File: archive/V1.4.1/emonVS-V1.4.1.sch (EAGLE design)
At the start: 47 parts, among them J7 RJ45 Jack, J8 TERMINAL_BLOCK_2P, J9 TERMINAL_BLOCK_5P, M1 275VAC, M2 275VAC, M3 275VAC, T1 ZMPT101B, T2 ZMPT101B, T3 ZMPT101B

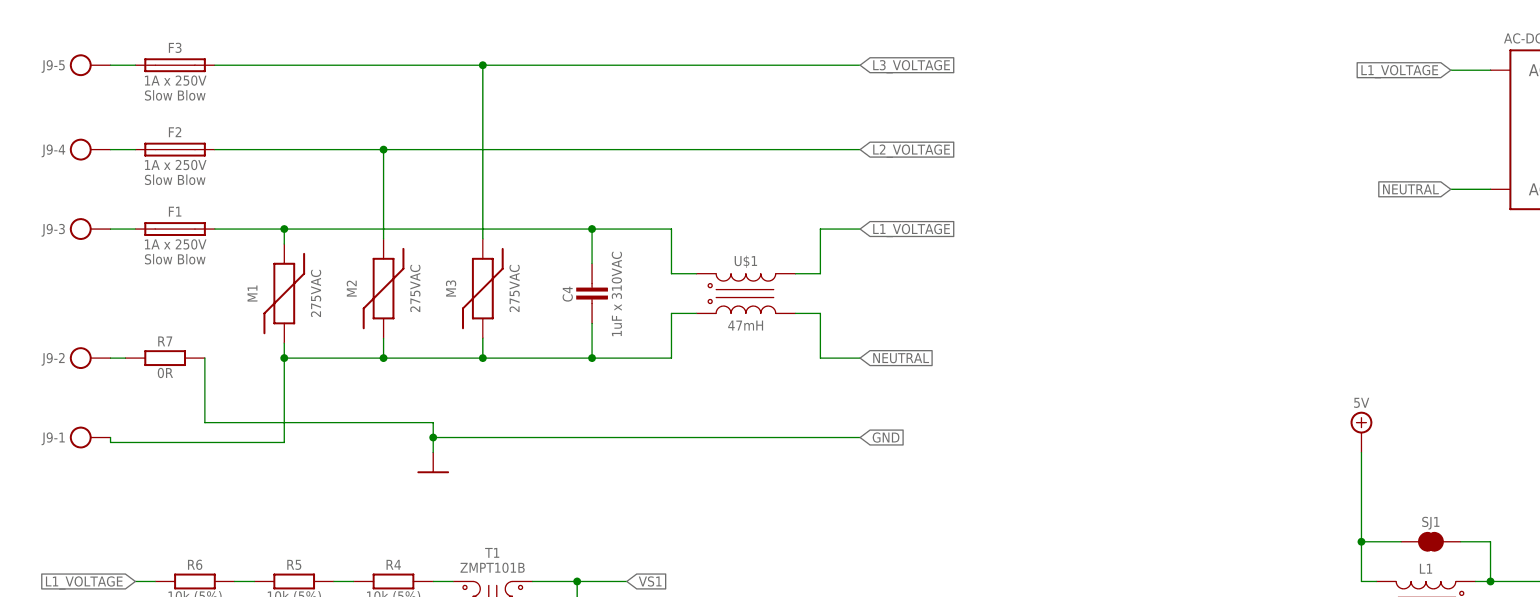
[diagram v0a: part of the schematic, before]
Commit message: 1.4.2
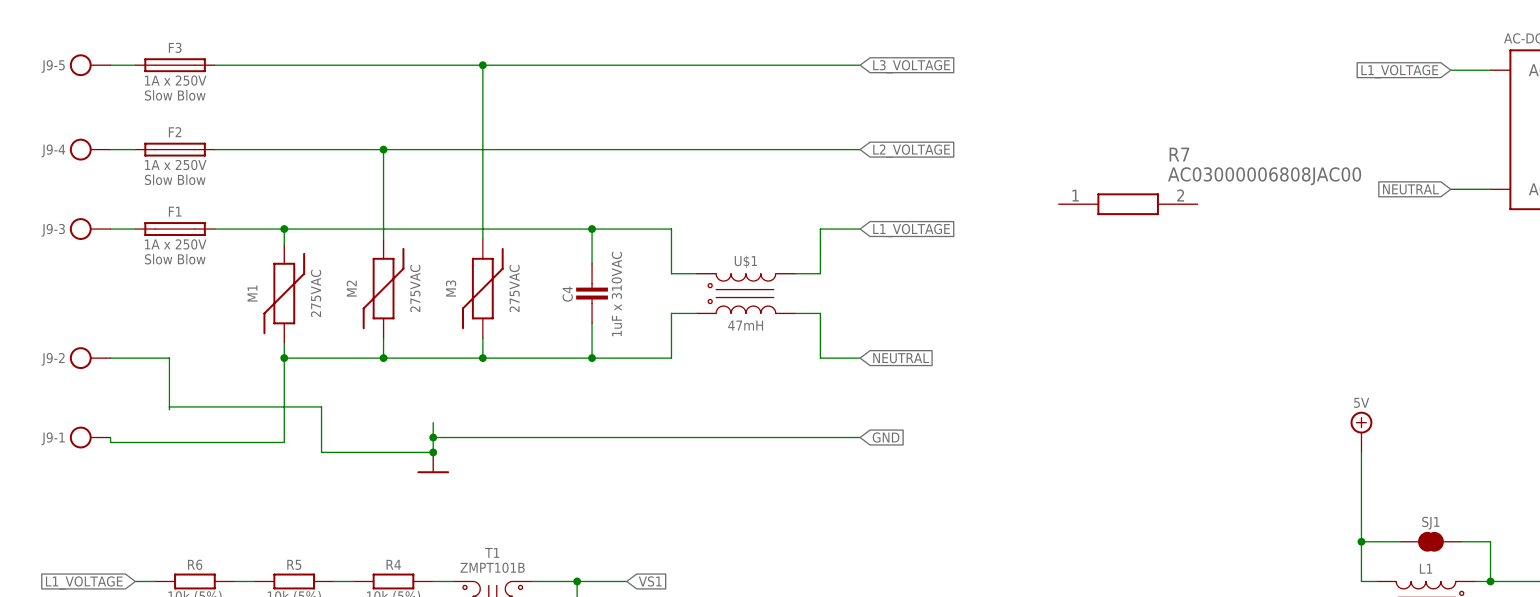
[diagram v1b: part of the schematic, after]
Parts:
- C5: device My-RLC:CP_SV-C -> My-RLC:CP_SV-D
- R7: value 0R -> AC03000006808JAC00; device My-RLC:R_1206 -> AC03000006808JAC00:AC03000006808JAC00; PN ERJ-H3GJ103V -> (none)
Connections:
- removed net N$20: J9-2.P$1, R7.2
- net GND: now also J9-2.P$1; no longer R7.1
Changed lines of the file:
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@@
 <setting verticaltext="up"/>
 </settings>
-<grid distance="0.025" unitdist="inch" unit="inch" style="lines" multiple="1" display="no" altdistance="0.01" altunitdist="inch" altunit="inch"/>
+<grid distance="0.1" unitdist="inch" unit="inch" style="lines" multiple="1" display="no" altdistance="0.01" altunitdist="inch" altunit="inch"/>
 <layers>
 <layer number="1" name="Top" color="59" fill="1" visible="no" active="no"/>
@@
 <attribute name="PN" value="GCM188R71C105KA64D"/>
 </part>
-<part name="C5" library="My-RLC" library_urn="urn:adsk.eagle:library:35509816" deviceset="CP_" device="SV-C" package3d_urn="urn:adsk.eagle:package:35509926/1" value="180uF x 6.3V">
+<part name="C5" library="My-RLC" library_urn="urn:adsk.eagle:library:35509816" deviceset="CP_" device="SV-D" package3d_urn="urn:adsk.eagle:package:35509947/1" value="180uF x 6.3V">
 <attribute name="PN" value="6SVPE180M"/>
 </part>
@@
 <part name="SUPPLY7" library="My-Supply" library_urn="urn:adsk.eagle:library:35531236" deviceset="0V" device=""/>
 <part name="SUPPLY8" library="My-Supply" library_urn="urn:adsk.eagle:library:35531236" deviceset="5V" device=""/>
-<part name="R7" library="My-RLC" library_urn="urn:adsk.eagle:library:35509816" deviceset="R_" device="1206" package3d_urn="urn:adsk.eagle:package:35509967/1" value="0R">
-<attribute name="PN" value="ERJ-H3GJ103V"/>
-</part>
+<part name="R7" library="AC03000006808JAC00" deviceset="AC03000006808JAC00" device=""/>
 </parts>
 <sheets>
@@
 <attribute name="VALUE" x="178.4096" y="119.38" size="1.27" layer="96" rot="MR0" align="center"/>
 </instance>
-<instance part="R7" gate="G$1" x="25.4" y="125.095" smashed="yes" rot="MR0">
-<attribute name="PN" x="25.4" y="125.095" size="1.778" layer="96" display="off"/>
-<attribute name="NAME" x="25.4" y="127.2286" size="1.27" layer="95" rot="MR0" align="center"/>
-<attribute name="VALUE" x="25.4" y="123.19" size="1.27" layer="96" rot="MR0" align="center"/>
+<instance part="R7" gate="G$1" x="139.7" y="144.78" smashed="yes">
+<attribute name="NAME" x="153.67" y="151.13" size="1.778" layer="95" align="center-left"/>
+<attribute name="VALUE" x="153.67" y="148.59" size="1.778" layer="96" align="center-left"/>
 </instance>
 </instances>
@@
 <wire x1="59.69" y1="114.935" x2="114.3" y2="114.935" width="0.1524" layer="91" grouprefs="THREE-PHASE_AC_NETWORK_INTERFACE"/>
 <wire x1="59.69" y1="113.03" x2="59.69" y2="114.935" width="0.1524" layer="91" grouprefs="THREE-PHASE_AC_NETWORK_INTERFACE"/>
-<pinref part="R7" gate="G$1" pin="1"/>
-<wire x1="30.48" y1="125.095" x2="30.48" y2="116.84" width="0.1524" layer="91"/>
-<wire x1="30.48" y1="116.84" x2="59.69" y2="116.84" width="0.1524" layer="91"/>
 <wire x1="59.69" y1="116.84" x2="59.69" y2="114.935" width="0.1524" layer="91"/>
 <junction x="59.69" y="114.935"/>
+<wire x1="59.69" y1="113.03" x2="45.406003125" y2="113.03" width="0.1524" layer="91"/>
+<wire x1="45.406003125" y1="113.03" x2="45.406003125" y2="118.84200625" width="0.1524" layer="91"/>
+<junction x="59.69" y="113.03"/>
+<wire x1="45.406003125" y1="118.84200625" x2="25.9462875" y2="118.84200625" width="0.1524" layer="91"/>
+<wire x1="25.9462875" y1="118.84200625" x2="25.9462875" y2="118.48188125" width="0.1524" layer="91"/>
+<pinref part="J9" gate="-2" pin="P$1"/>
+<wire x1="25.9462875" y1="118.84200625" x2="25.9462875" y2="125.095" width="0.1524" layer="91"/>
+<wire x1="25.9462875" y1="125.095" x2="18.415" y2="125.095" width="0.1524" layer="91"/>
 </segment>
 <segment>
@@
 </segment>
 </net>
-<net name="N$20" class="0">
-<segment>
-<pinref part="J9" gate="-2" pin="P$1"/>
-<pinref part="R7" gate="G$1" pin="2"/>
-<wire x1="18.415" y1="125.095" x2="20.32" y2="125.095" width="0.1524" layer="91"/>
-</segment>
-</net>
